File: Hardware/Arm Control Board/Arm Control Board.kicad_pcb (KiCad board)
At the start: 2 copper layers, 99 parts, among them P1 Servo 1, P10 UIM240XX_Stepper_Conn, P11 Battery, P12 SyRen, P13 Raspberry Pi, P2 Shoulder Feedback, P3 Servo 2, P4 Servo 3, P5 Elbow Feedback, P6 Servo 4, P7 RS485, P8 ST_SWD_Connector, P9 Servo 5, U1 STM32F401RCT6, U2 SN75176BDR, U3 74LVCH244APW, U4 AOZ1280CI, U5 AOZ1280CI, U6 AP65552SP-13, U7 AP65552SP-13, U8 AP65552SP-13, U9 AP65552SP-13, X1 24MHz

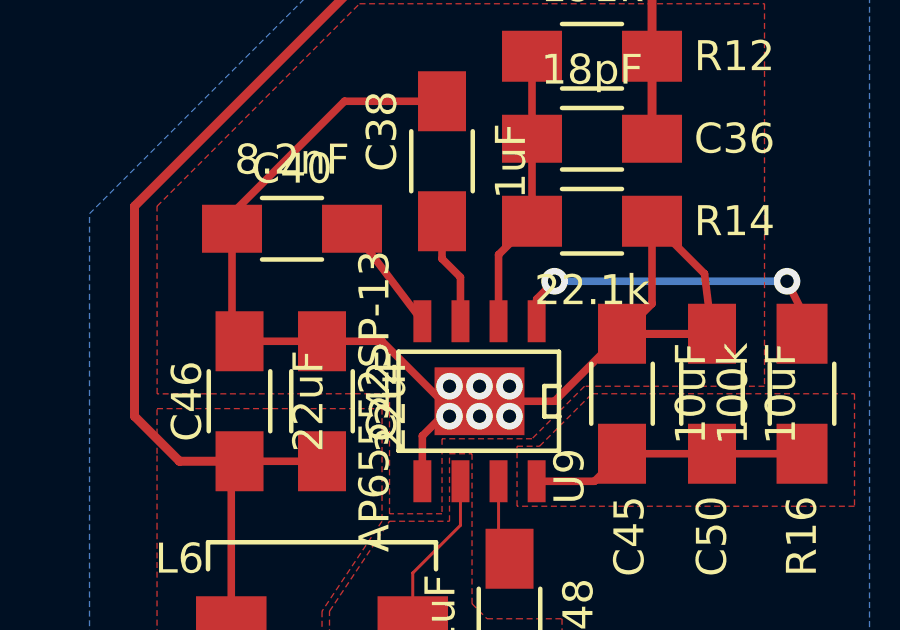
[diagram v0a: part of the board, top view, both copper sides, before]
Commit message: more vias but to be honest the situation is a mess
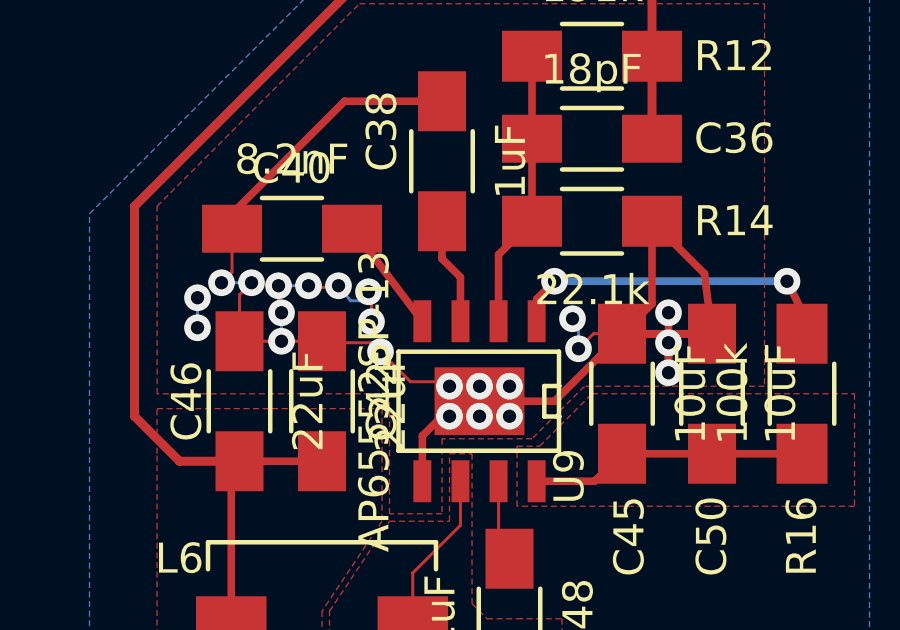
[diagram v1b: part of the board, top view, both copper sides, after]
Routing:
- net GND: track 158.6 -> 173.8 mm, vias 6 -> 21
- net (no net): track 0.00 -> 1.00 mm, vias 0 -> 2
